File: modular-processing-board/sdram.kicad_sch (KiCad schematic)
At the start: 18 parts, among them U301 W9825G6KH-6, U302 W9825G6KH-6

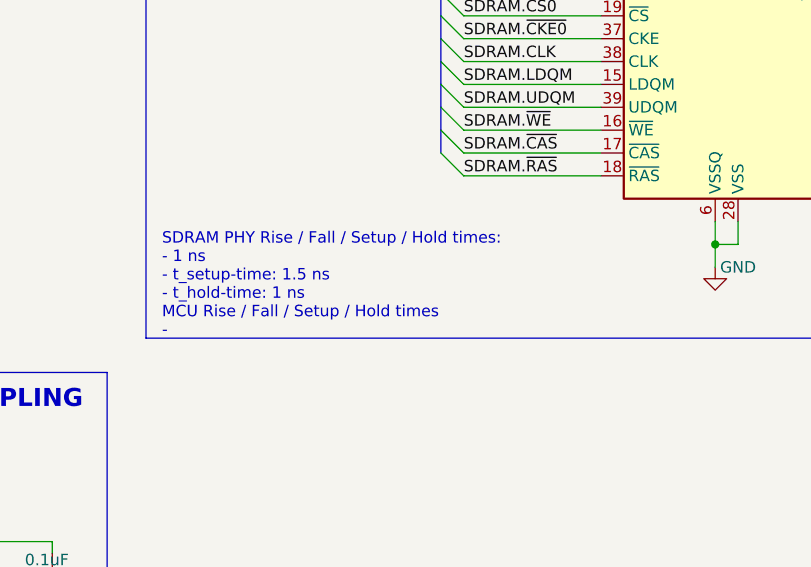
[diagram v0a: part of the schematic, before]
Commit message: minor change in fw
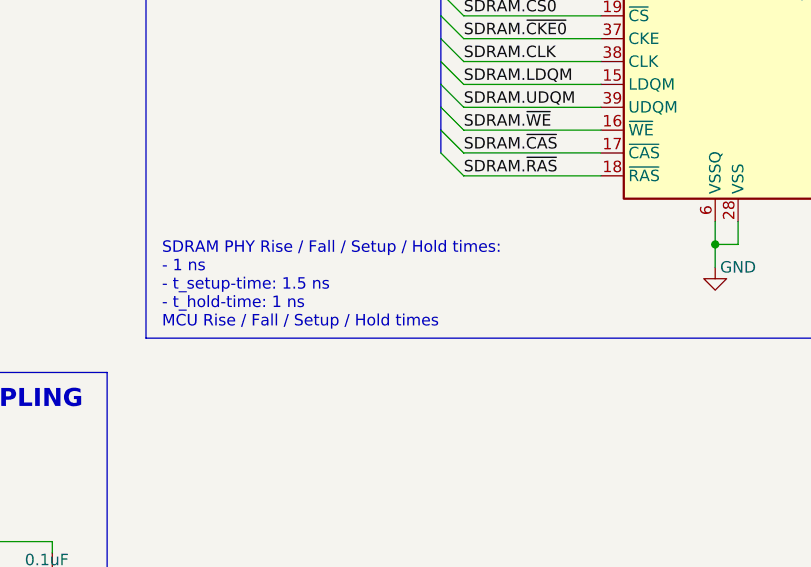
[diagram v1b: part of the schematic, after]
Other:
- note added: "SDRAM PHY Rise / Fall / Setup / Hold times: - 1 ns - t_setup-time: 1.5 ns - t_hold-time: 1 ns MCU Rise / Fall / Setup / Hold times"
- note removed: "SDRAM PHY Rise / Fall / Setup / Hold times: - 1 ns - t_setup-time: 1.5 ns - t_hold-time: 1 ns MCU Rise / Fall / Setup / Hold times -"
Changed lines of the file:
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@@
 		)
 	)
-	(text "SDRAM PHY Rise / Fall / Setup / Hold times:\n- 1 ns\n- t_setup-time: 1.5 ns\n- t_hold-time: 1 ns\nMCU Rise / Fall / Setup / Hold times\n- "
+	(text "SDRAM PHY Rise / Fall / Setup / Hold times:\n- 1 ns\n- t_setup-time: 1.5 ns\n- t_hold-time: 1 ns\nMCU Rise / Fall / Setup / Hold times"
 		(exclude_from_sim no)
 		(at 93.472 121.412 0)
